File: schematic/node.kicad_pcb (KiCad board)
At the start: 2 copper layers, 12 parts, among them IC1 ATMEGA328P-P, P1 NRF24L01, P2 CONN_01X06, P3 CONN_01X02

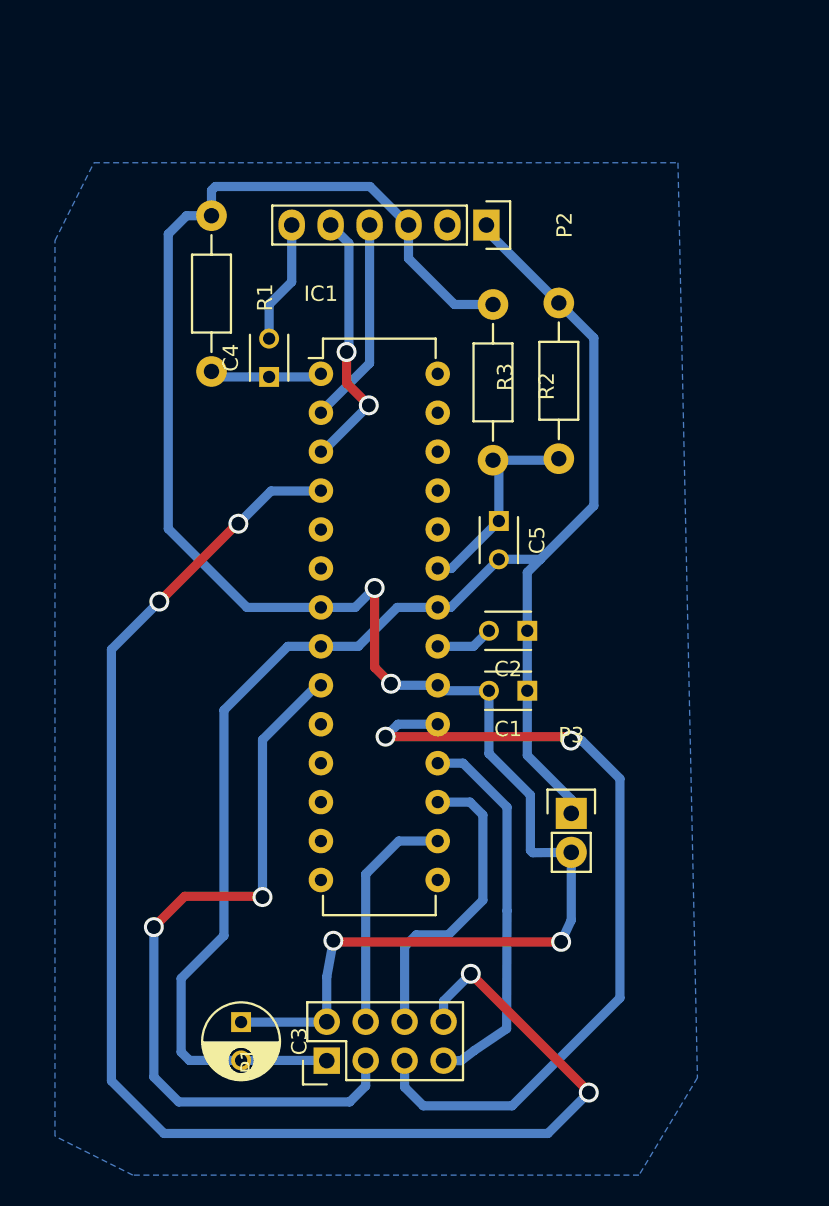
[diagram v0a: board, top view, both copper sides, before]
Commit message: add kicad design files
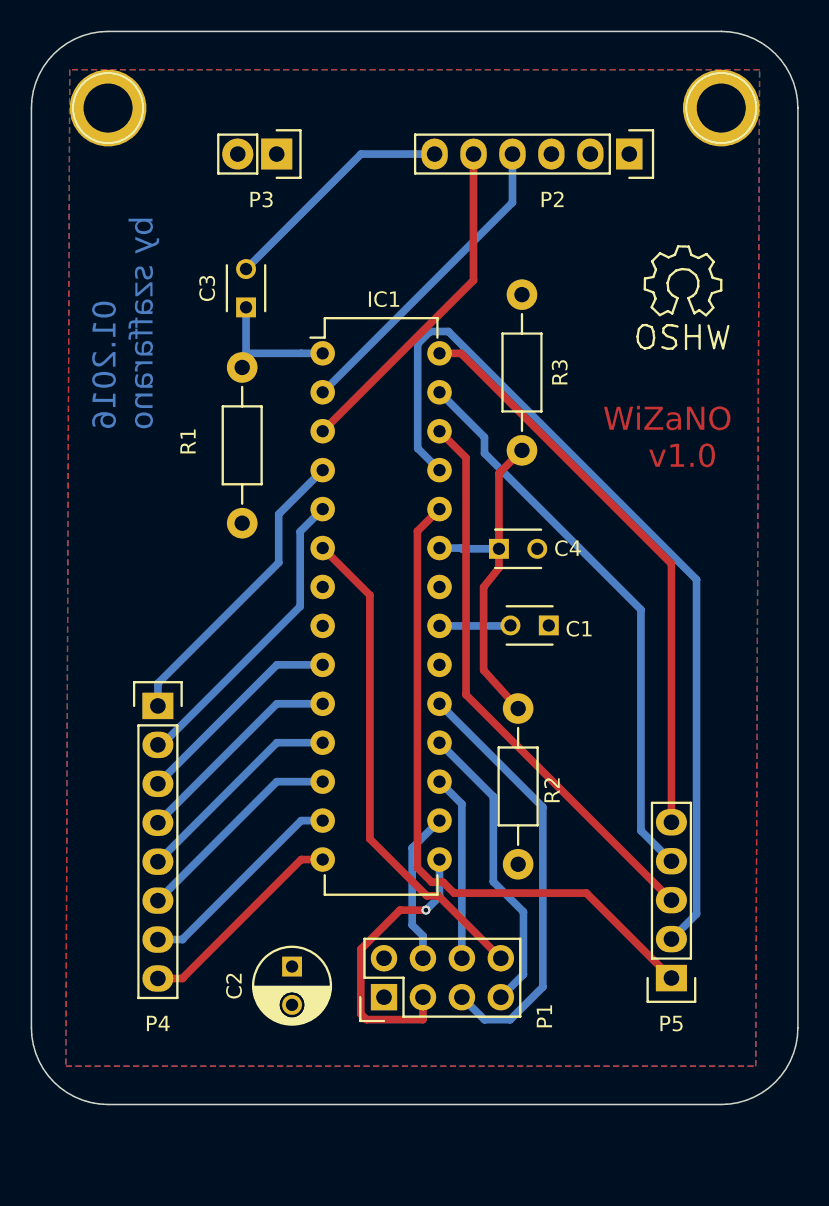
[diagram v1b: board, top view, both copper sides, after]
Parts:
- removed C5: 0.1 uF, Capacitors_ThroughHole:C_Disc_D3_P2.5
- added P4: HEADER_LEFT, Pin_Headers:Pin_Header_Straight_1x08, F.Cu at (150.2, 127.0)
- added P5: HEADER_RIGHT, Pin_Headers:Pin_Header_Straight_1x05, F.Cu at (183.8, 144.8)
- added REF**: 1pin, Connect:1pin, F.Cu at (187.0, 88.0)
- added REF**: 1pin, Connect:1pin, F.Cu at (147.0, 88.0)
- added REF**: Symbol_OSHW-Logo_SilkScreen, Symbols:Symbol_OSHW-Logo_SilkScreen, F.Cu at (184.5, 99.5)
- C2: value 0.1 uF -> 4.7 uF; footprint Capacitors_ThroughHole:C_Disc_D3_P2.5 -> Capacitors_ThroughHole:C_Radial_D5_L11_P2.5
- C3: value 4.7 uF -> 0.1 uF; footprint Capacitors_ThroughHole:C_Radial_D5_L6_P2.5 -> Capacitors_ThroughHole:C_Disc_D3_P2.5
- P2: value CONN_01X06 -> FTDI
- P3: value CONN_01X02 -> POWER
- moved P3 47.1 mm to (158.0, 91.0), turned to 270 degrees
- moved C3 46.6 mm to (156.0, 101.0), turned to 90 degrees
- moved C2 26.7 mm to (159.0, 144.0), turned to 270 degrees
- moved R2 26.4 mm to (173.8, 132.2), turned to 90 degrees
- moved C4 18.7 mm to (172.5, 116.8), turned to 0 degrees
- moved P2 10.4 mm to (181.0, 91.0)
- moved R1 10.1 mm to (155.8, 110.0), turned to 90 degrees
- moved P1 5.58 mm to (165.0, 146.0)
- moved C1 4.48 mm to (175.8, 121.8)
- moved R3 2.46 mm to (174.0, 105.2)
- moved IC1 1.34 mm to (161.0, 104.0)
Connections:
- net /RX renamed RX
- net /TX renamed TX
- C1 pad 2: +3V3 -> Net-(C1-Pad2)
- C2 pad 1: GND -> +3V3
- C2 pad 2: Net-(C2-Pad2) -> GND
- C3 pad 1: +3V3 -> Net-(C3-Pad1)
- C3 pad 2: GND -> DTR
- C4 pad 2: /DTR -> GND
- IC1 pad 1: Net-(C4-Pad1) -> Net-(C3-Pad1)
- IC1 pad 10: Net-(IC1-Pad10) -> PB7
- IC1 pad 11: Net-(IC1-Pad11) -> PD5
- IC1 pad 12: Net-(IC1-Pad12) -> PD6
- IC1 pad 13: Net-(IC1-Pad13) -> PD7
- IC1 pad 14: Net-(IC1-Pad14) -> PB0
- IC1 pad 21: Net-(C2-Pad2) -> Net-(C1-Pad2)
- IC1 pad 23: Net-(C5-Pad1) -> Net-(C4-Pad1)
- IC1 pad 24: Net-(IC1-Pad24) -> PC1
- IC1 pad 25: Net-(IC1-Pad25) -> PC2
- IC1 pad 26: Net-(IC1-Pad26) -> PC3
- IC1 pad 27: Net-(IC1-Pad27) -> PC4
- IC1 pad 28: Net-(IC1-Pad28) -> PC5
- IC1 pad 4: Net-(IC1-Pad4) -> PD2
- IC1 pad 5: Net-(IC1-Pad5) -> PD3
- IC1 pad 9: Net-(IC1-Pad9) -> PB6
- P1 pad 3: Net-(IC1-Pad9) -> Net-(IC1-Pad15)
- P1 pad 8: Net-(IC1-Pad4) -> Net-(IC1-Pad6)
- P2 pad 6: /DTR -> DTR
- R1 pad 2: Net-(C4-Pad1) -> Net-(C3-Pad1)
- R2 pad 2: Net-(C5-Pad1) -> Net-(C4-Pad1)
- R3 pad 1: Net-(C5-Pad1) -> Net-(C4-Pad1)
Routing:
- net +3V3: track 122.7 -> 0.00 mm, vias 4 -> 0
- net GND: track 102.2 -> 0.00 mm
- net Net-(IC1-Pad4): track 94.6 -> 0.00 mm, vias 4 -> 0
- net PC2: track 0.00 -> 58.2 mm
- net Net-(IC1-Pad9): track 49.8 -> 0.00 mm, vias 2 -> 0
- net PC1: track 0.00 -> 43.5 mm
- net PC5: track 0.00 -> 37.7 mm
- net PC4: track 0.00 -> 36.9 mm
- net PC3: track 0.00 -> 36.9 mm
- net Net-(IC1-Pad6): track 0.00 -> 32.0 mm
- net Net-(IC1-Pad19): track 53.7 -> 28.0 mm, vias 2 -> 0
- net PD3: track 0.00 -> 20.0 mm
- net PD2: track 0.00 -> 19.8 mm
- net Net-(IC1-Pad15): track 0.00 -> 18.9 mm, vias 0 -> 1
- net DTR: track 0.00 -> 15.4 mm
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- added copper zone on F.Cu, net +3V3
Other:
- board outline added: 50 x 70 mm
- net class Default: clearance 0.5 -> 0.35; trace_width 0.6 -> 0.5; via_dia 1.3 -> 0.6; via_drill 0.9 -> 0.4
- rule pad_to_mask_clearance: 0.2 -> 0
- rule trace_clearance: 0.5 -> 0.35
- board text added: "01.2016 by szaffarano"
- board text added: "WiZaNO v1.0"
